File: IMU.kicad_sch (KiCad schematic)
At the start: 11 parts, among them U1 ICM-42688-P

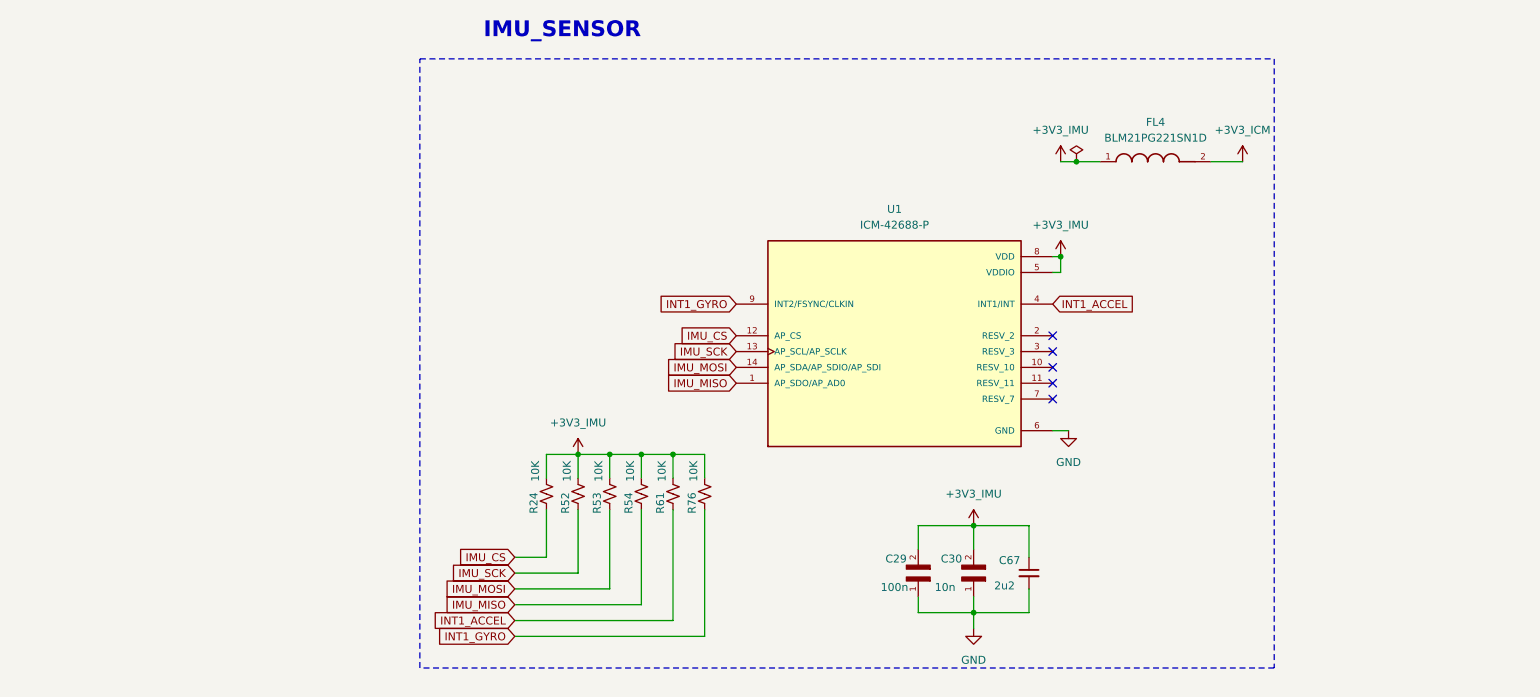
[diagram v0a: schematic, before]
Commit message: can
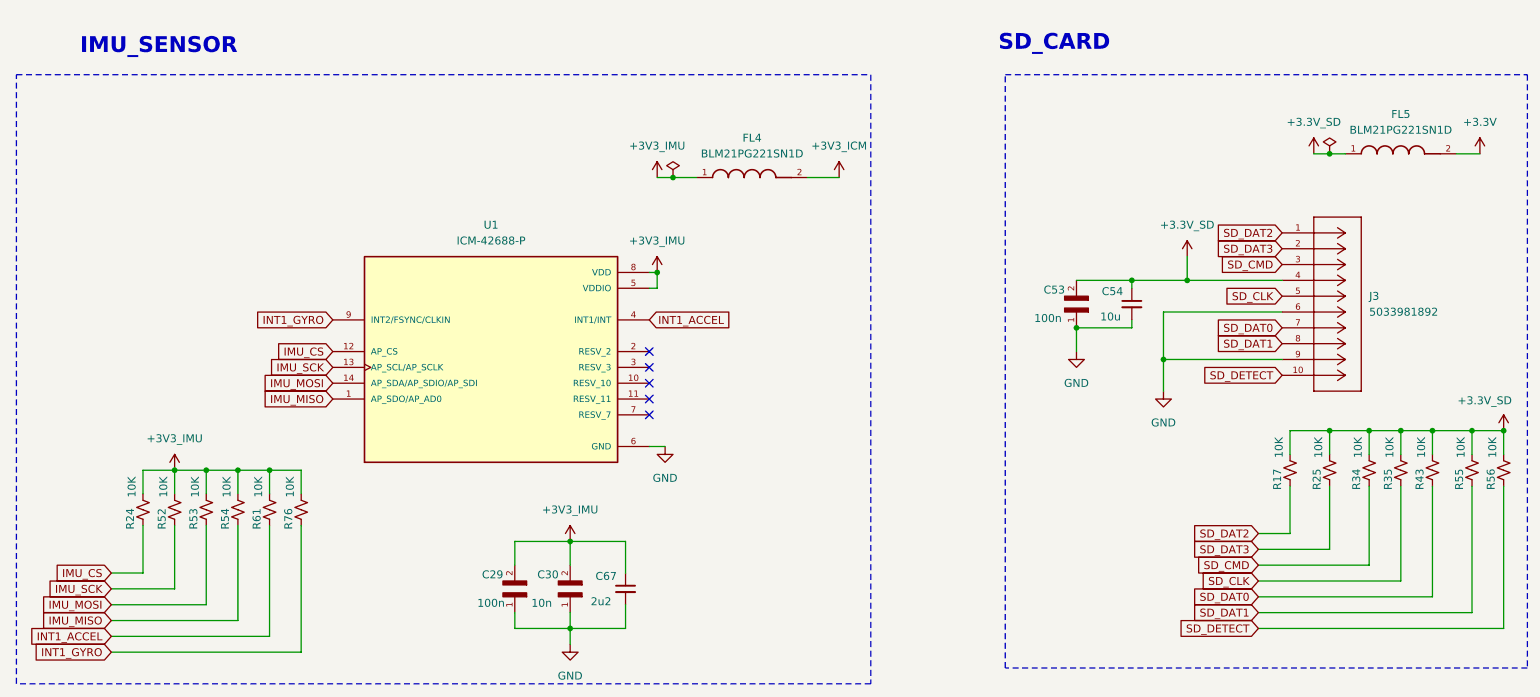
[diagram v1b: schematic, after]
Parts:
- added C53: 100n, Capacitor_SMD:C_0402_1005Metric, symbol C0402C104K4RAC:C0402C104K4RAC
- added C54: 10u, Capacitor_SMD:C_0805_2012Metric, symbol Device:C_Small
- added FL5: BLM21PG221SN1D, BLM21PG221SN1D:BEADC2012X105N, symbol BLM21PG221SN1D:BLM21PG221SN1D
- added J3: 5033981892, GNSS:CONN_503398-1892_MOL, symbol 5033981892:5033981892
- added R17, R25, R34, R35, R43, R55, R56: 10K, Resistor_SMD:R_0402_1005Metric, symbol Device:R_Small_US
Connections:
- net GND: now also C53.1, C54.2, J3.6, J3.9
- new net +3.3V: FL5.2
- new net +3.3V_SD: C53.2, C54.1, FL5.1, J3.4, R17.2, R25.2, R34.2, R35.2, R43.2, R55.2, R56.2
- new net SD_CLK: J3.5, R35.1
- new net SD_CMD: J3.3, R34.1
- new net SD_DAT0: J3.7, R43.1
- new net SD_DAT1: J3.8, R55.1
- new net SD_DAT2: J3.1, R17.1
- new net SD_DAT3: J3.2, R25.1
- new net SD_DETECT: J3.10, R56.1
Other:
- note added: "SD_CARD"
- moved on the sheet: C29, C30, C67, FL4, R24, R52, R53, R54, R61, R76, U1
